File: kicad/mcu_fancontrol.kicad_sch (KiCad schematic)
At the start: 48 parts, among them J1 Vin, J10 NTC1, J11 NTC2, J2 SWIM, J3 UART, J4 Output1, J5 Output2, J6 1-Wire, J7 I2C, J8 I2C, J9 1-Wire, Q1 BSS138, Q2 AO3401A, U1 STM8S003F3P, U2 LM75C, U3 L78L05_SOT89

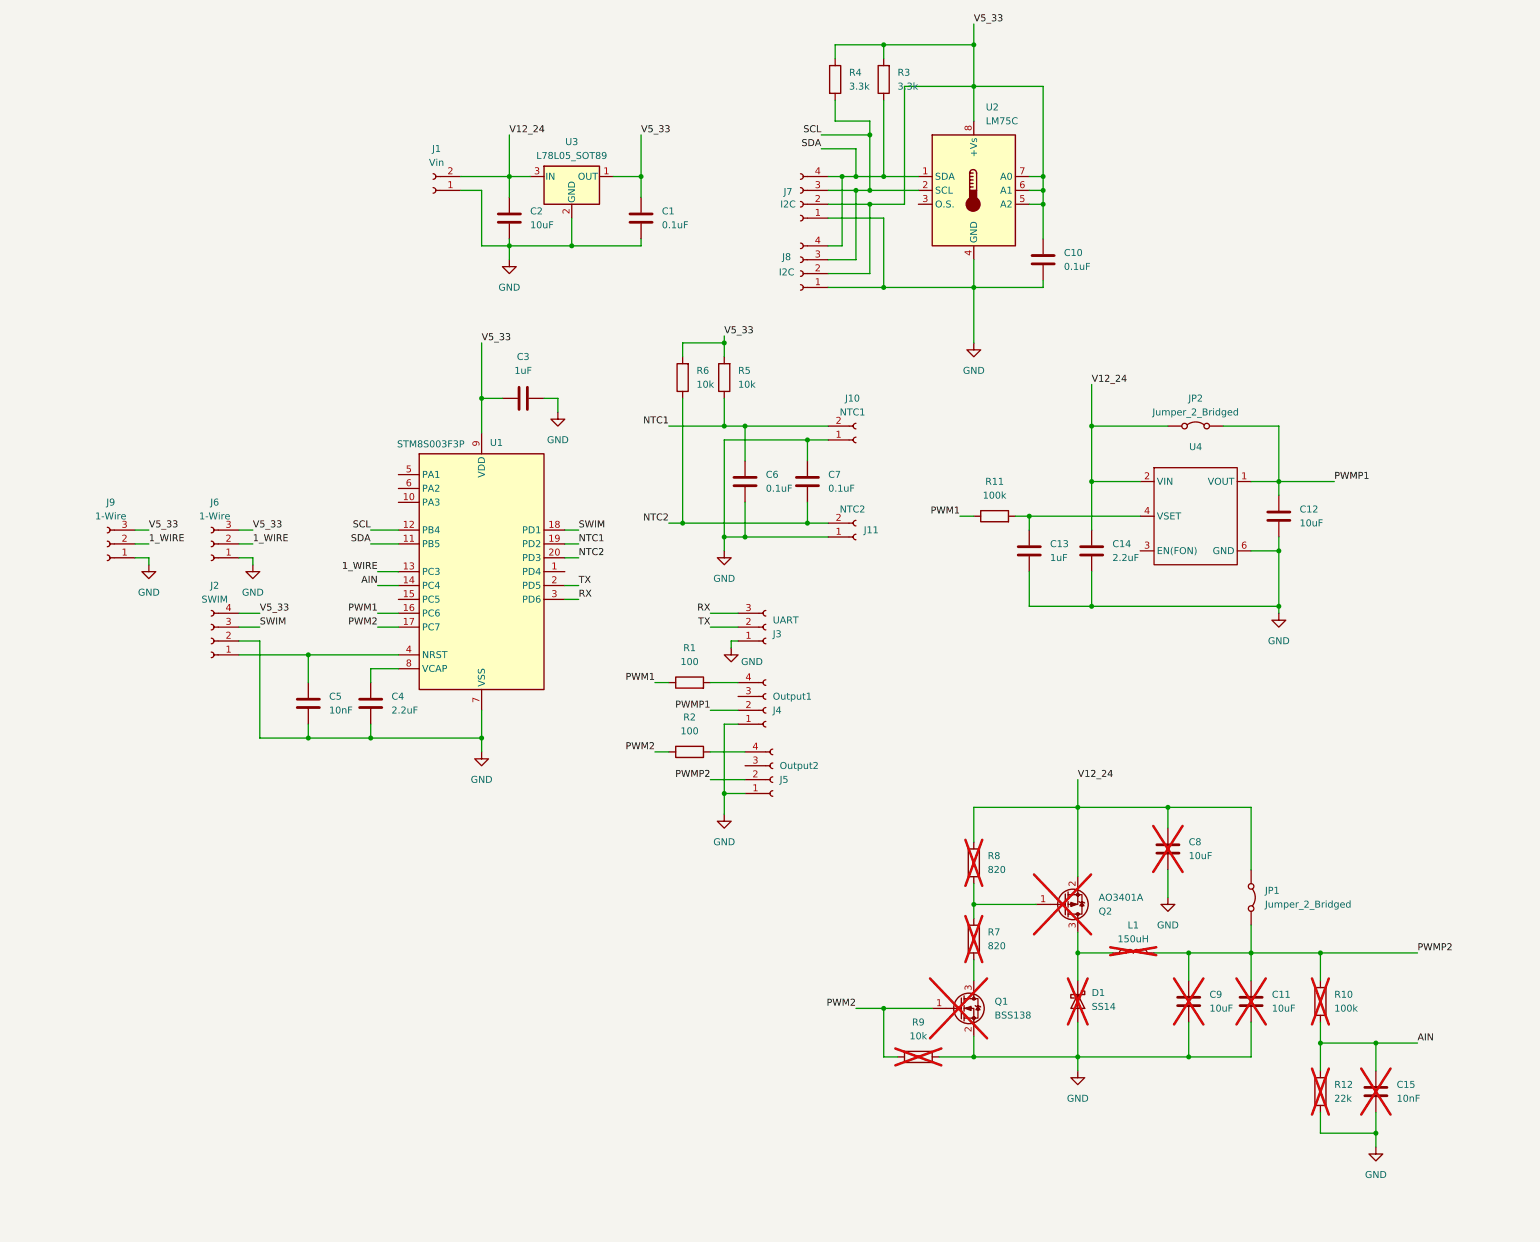
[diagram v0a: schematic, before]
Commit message: Add new PCB design
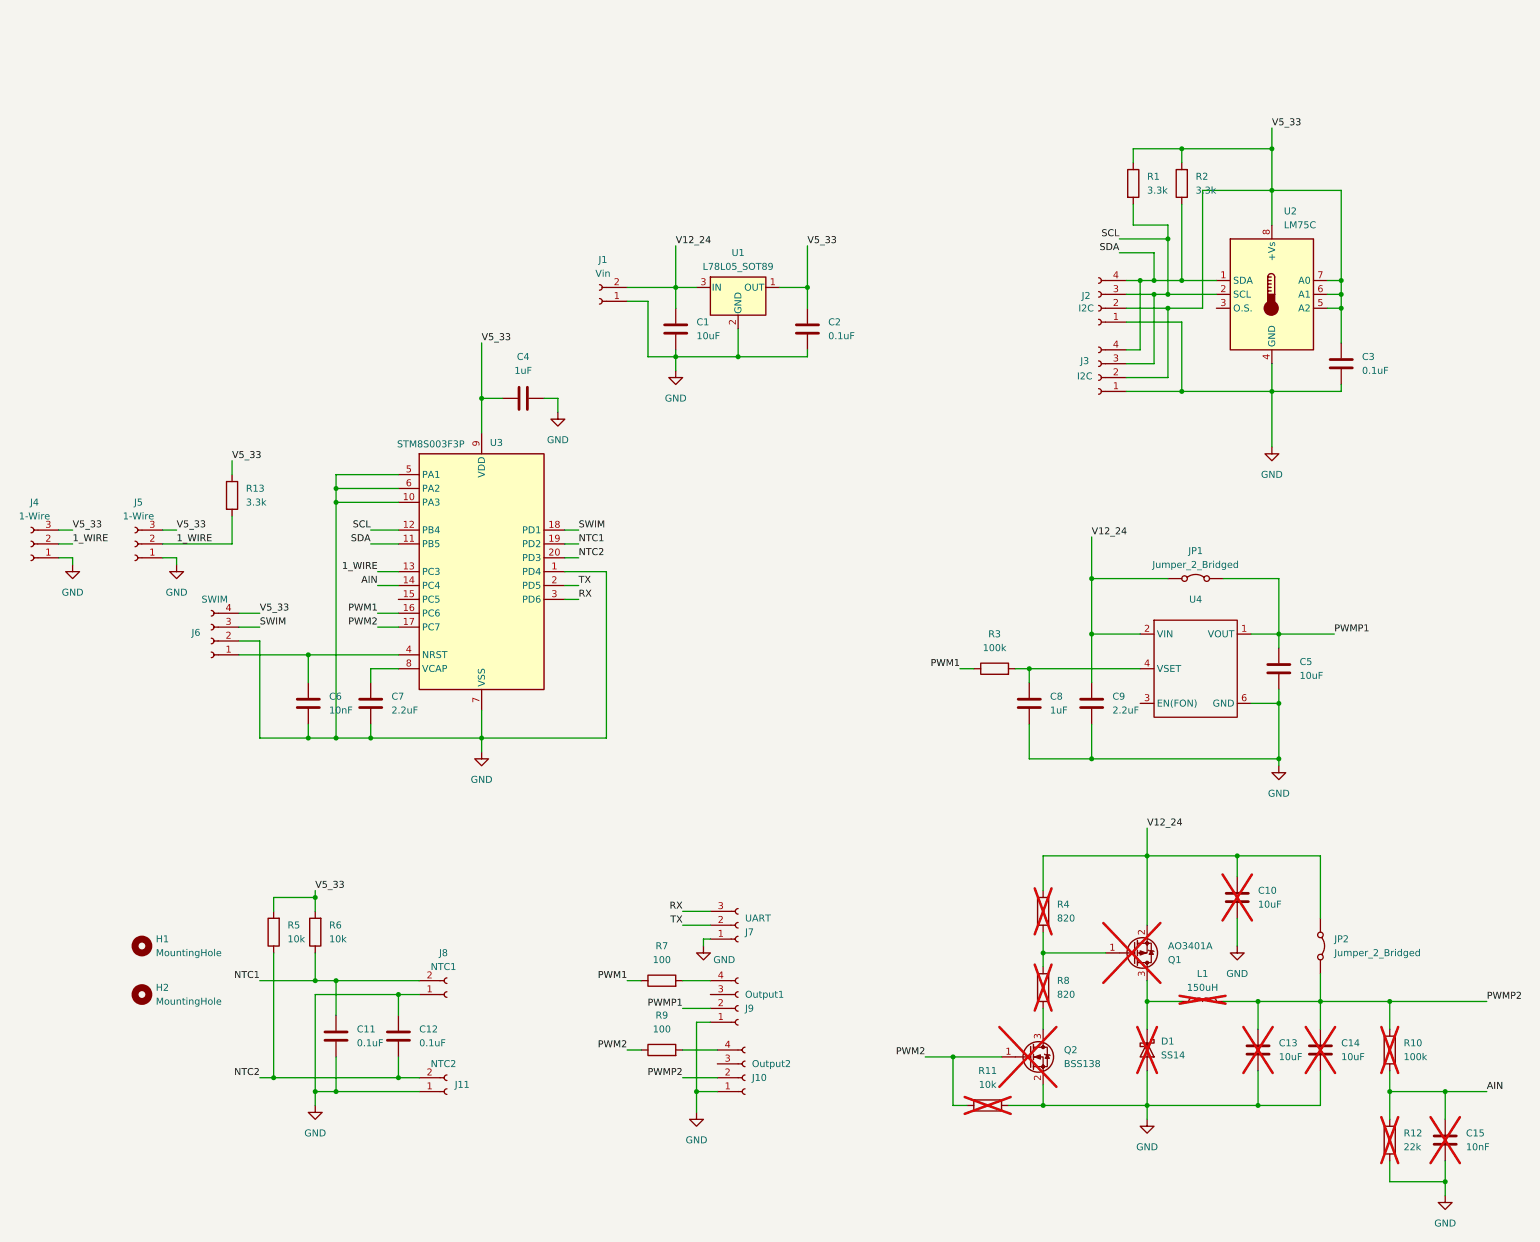
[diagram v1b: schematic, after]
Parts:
- added H1, H2: MountingHole, MountingHole:MountingHole_2.7mm_M2.5, symbol Mechanical:MountingHole
- added R13: 3.3k, Resistor_SMD:R_0603_1608Metric, symbol Device:R
- C1: renamed from C2; footprint (none) -> Capacitor_SMD:C_1206_3216Metric
- C10: renamed from C8; footprint (none) -> Capacitor_SMD:C_1206_3216Metric
- C11: renamed from C6; footprint (none) -> Capacitor_SMD:C_0603_1608Metric
- C12: renamed from C7; footprint (none) -> Capacitor_SMD:C_0603_1608Metric
- C13: renamed from C9; footprint (none) -> Capacitor_SMD:C_1206_3216Metric
- C14: renamed from C11; footprint (none) -> Capacitor_SMD:C_1206_3216Metric
- C15: footprint (none) -> Capacitor_SMD:C_0603_1608Metric
- C2: renamed from C1; footprint (none) -> Capacitor_SMD:C_0603_1608Metric
- C3: renamed from C10; footprint (none) -> Capacitor_SMD:C_0603_1608Metric
- C4: renamed from C3; footprint (none) -> Capacitor_SMD:C_0603_1608Metric
- C5: renamed from C12; footprint (none) -> Capacitor_SMD:C_1206_3216Metric
- C6: renamed from C5; footprint (none) -> Capacitor_SMD:C_0603_1608Metric
- C7: renamed from C4; footprint (none) -> Capacitor_SMD:C_0603_1608Metric
- C8: renamed from C13; footprint (none) -> Capacitor_SMD:C_0603_1608Metric
- C9: renamed from C14; footprint (none) -> Capacitor_SMD:C_0603_1608Metric
- J1: footprint (none) -> Connector_Wire:SolderWire-0.5sqmm_1x02_P4.8mm_D0.9mm_OD2.3mm
- J10: renamed from J5; footprint (none) -> Connector:FanPinHeader_1x04_P2.54mm_Vertical
- J11: footprint (none) -> Connector_PinHeader_2.54mm:PinHeader_1x02_P2.54mm_Vertical
- J2: renamed from J7; footprint (none) -> Connector_PinSocket_2.54mm:PinSocket_1x04_P2.54mm_Vertical
- J3: renamed from J8; footprint (none) -> Connector_PinSocket_2.54mm:PinSocket_1x04_P2.54mm_Vertical
- J4: renamed from J9; footprint (none) -> Connector_PinSocket_2.54mm:PinSocket_1x03_P2.54mm_Vertical
- J5: renamed from J6; footprint (none) -> Connector_PinSocket_2.54mm:PinSocket_1x03_P2.54mm_Vertical
- J6: renamed from J2; footprint (none) -> Connector_PinSocket_2.54mm:PinSocket_1x04_P2.54mm_Vertical
- J7: renamed from J3; footprint (none) -> Connector_PinSocket_2.54mm:PinSocket_1x03_P2.54mm_Vertical
- J8: renamed from J10; footprint (none) -> Connector_PinHeader_2.54mm:PinHeader_1x02_P2.54mm_Vertical
- J9: renamed from J4; footprint (none) -> Connector:FanPinHeader_1x04_P2.54mm_Vertical
- JP1: renamed from JP2; footprint (none) -> Jumper:SolderJumper-2_P1.3mm_Open_RoundedPad1.0x1.5mm
- JP2: renamed from JP1; footprint (none) -> Jumper:SolderJumper-2_P1.3mm_Open_RoundedPad1.0x1.5mm
- L1: footprint (none) -> Inductor_THT:L_Radial_D7.0mm_P3.00mm
- R1: renamed from R4; footprint (none) -> Resistor_SMD:R_0603_1608Metric
- R10, R12: footprint (none) -> Resistor_SMD:R_0603_1608Metric
- R11: renamed from R9; footprint (none) -> Resistor_SMD:R_0603_1608Metric
- R2: renamed from R3; footprint (none) -> Resistor_SMD:R_0603_1608Metric
- R3: renamed from R11; footprint (none) -> Resistor_SMD:R_0603_1608Metric
- R4: renamed from R8; footprint (none) -> Resistor_SMD:R_1206_3216Metric
- R5: renamed from R6; footprint (none) -> Resistor_SMD:R_0603_1608Metric
- R6: renamed from R5; footprint (none) -> Resistor_SMD:R_0603_1608Metric
- R7: renamed from R1; footprint (none) -> Resistor_SMD:R_0603_1608Metric
- R8: renamed from R7; footprint (none) -> Resistor_SMD:R_1206_3216Metric
- R9: renamed from R2; footprint (none) -> Resistor_SMD:R_0603_1608Metric
- renumbered Q2 to Q1, Q1 to Q2, U3 to U1, U1 to U3
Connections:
- net 1_WIRE: now also R13.2
- net GND: now also U3.1 (PD4), U3.10 (PA3), U3.5 (PA1), U3.6 (PA2), U4.9 (PAD)
- net V5_33: now also R13.1
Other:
- moved on the sheet: C1, C10, C11, C12, C13, C14, C15, C2, C3, C5, C8, C9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
